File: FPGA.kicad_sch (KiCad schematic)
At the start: 1 part, among them U501 ICE40-HX8K_Breakout_Board

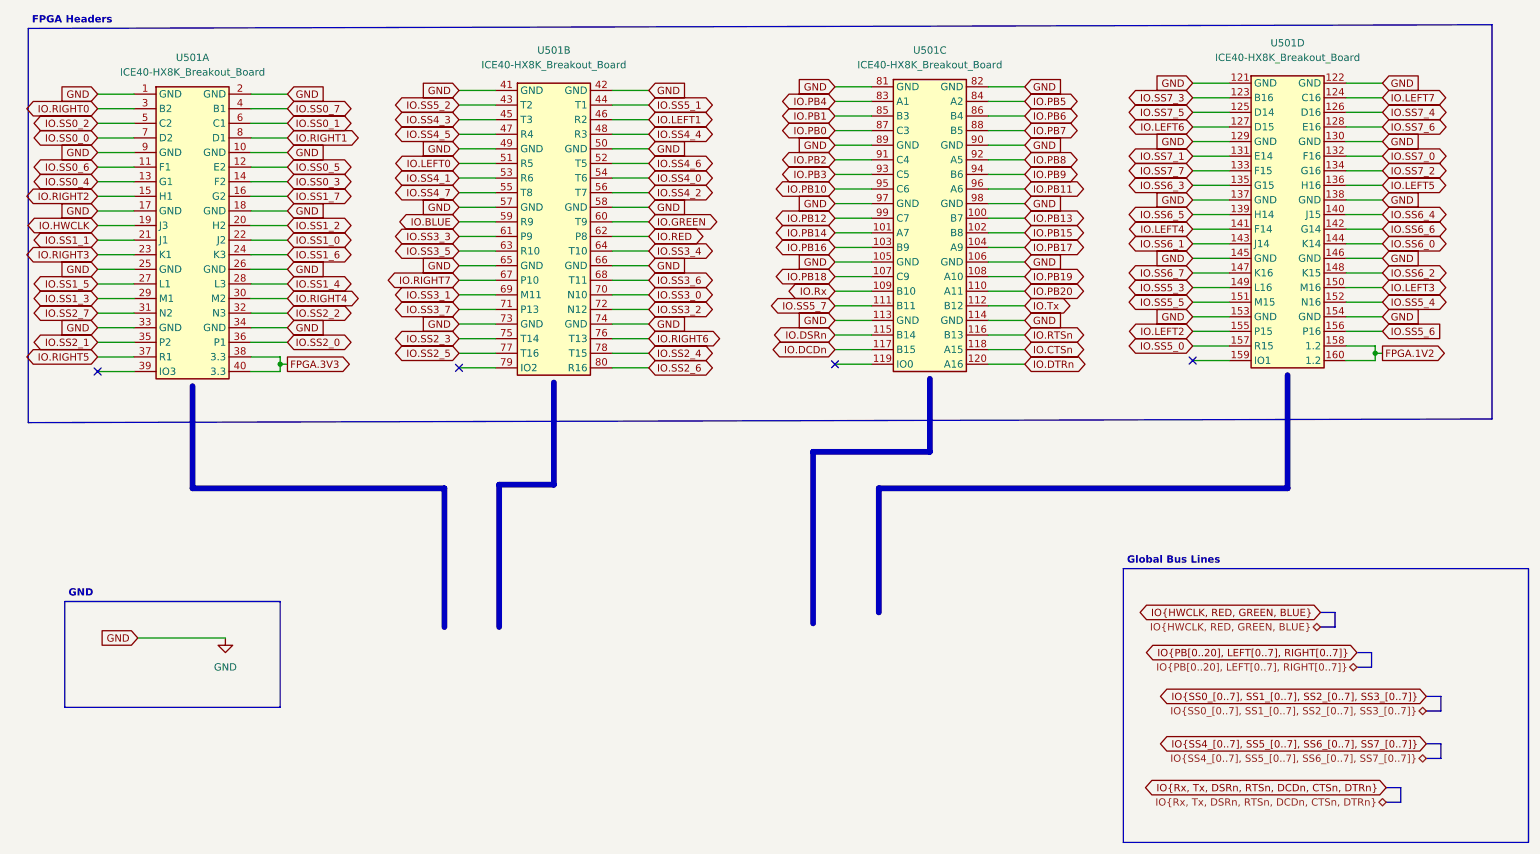
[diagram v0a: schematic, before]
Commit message: Complete Design
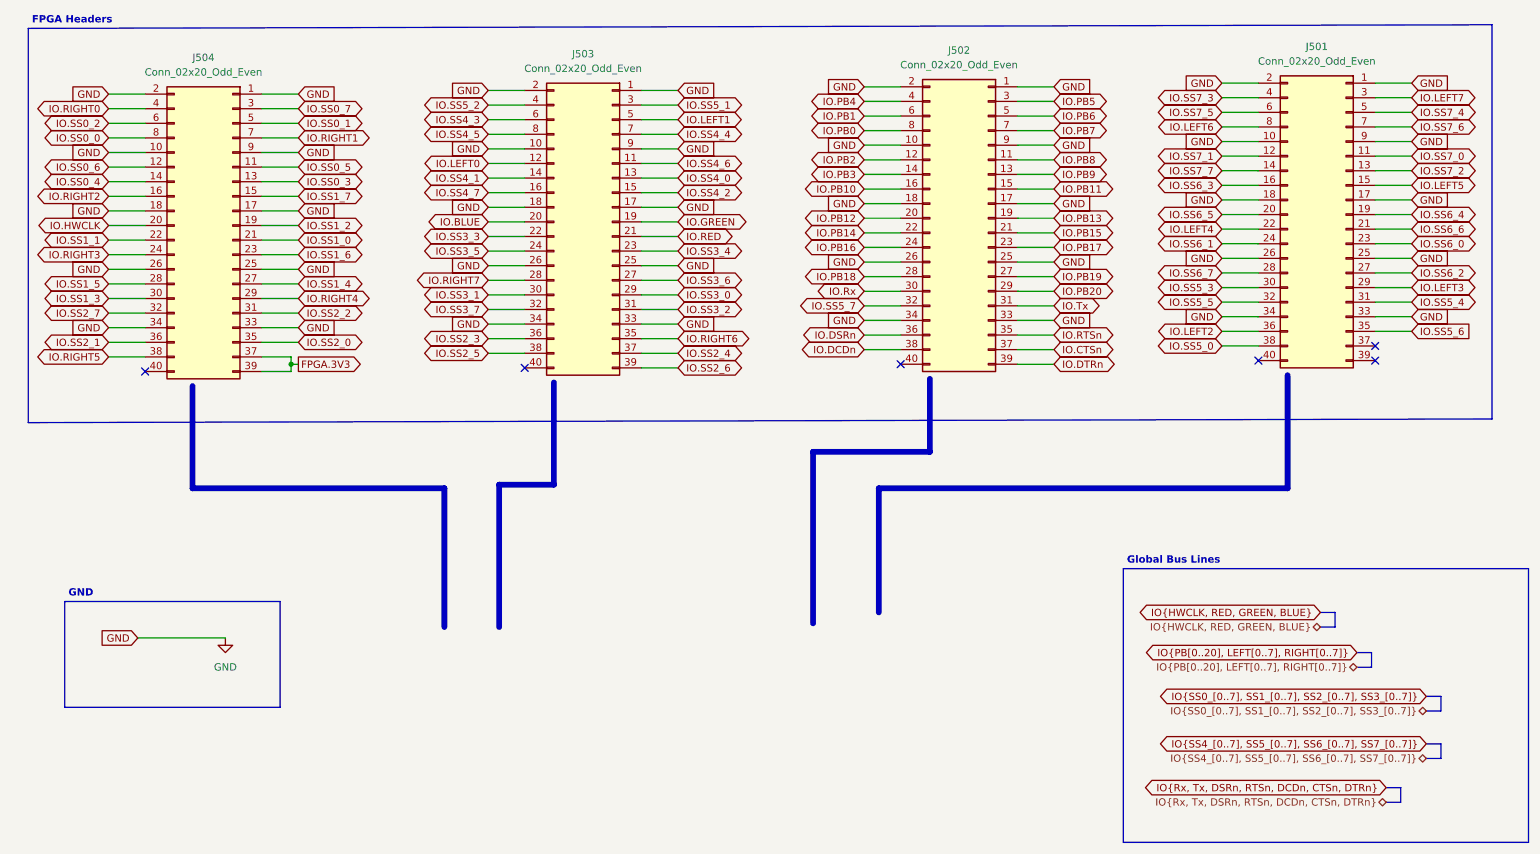
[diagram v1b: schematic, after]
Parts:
- removed U501: ICE40-HX8K_Breakout_Board, ECELab_Footprints:ICE40-HX8K Breakout Board, symbol ECELab_PartsLibrary:ICE40-HX8K_Breakout_Board
- added J501, J502, J503, J504: Conn_02x20_Odd_Even, Connector_PinHeader_2.54mm:PinHeader_2x20_P2.54mm_Vertical, symbol Connector_Generic:Conn_02x20_Odd_Even
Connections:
- net FPGA.3V3: now also J504.37 (Pin_37), J504.39 (Pin_39)
- net GND: now also J501.1 (Pin_1), J501.10 (Pin_10), J501.17 (Pin_17), J501.18 (Pin_18), J501.2 (Pin_2), J501.25 (Pin_25), J501.26 (Pin_26), J501.33 (Pin_33), J501.34 (Pin_34), J501.9 (Pin_9), J502.1 (Pin_1), J502.10 (Pin_10), J502.17 (Pin_17), J502.18 (Pin_18), J502.2 (Pin_2), J502.25 (Pin_25), J502.26 (Pin_26), J502.33 (Pin_33), J502.34 (Pin_34), J502.9 (Pin_9), J503.1 (Pin_1), J503.10 (Pin_10), J503.17 (Pin_17), J503.18 (Pin_18), J503.2 (Pin_2), J503.25 (Pin_25), J503.26 (Pin_26), J503.33 (Pin_33), J503.34 (Pin_34), J503.9 (Pin_9), J504.1 (Pin_1), J504.10 (Pin_10), J504.17 (Pin_17), J504.18 (Pin_18), J504.2 (Pin_2), J504.25 (Pin_25), J504.26 (Pin_26), J504.33 (Pin_33), J504.34 (Pin_34), J504.9 (Pin_9)
- net IO.BLUE: now also J503.20 (Pin_20)
- net IO.CTSn: now also J502.37 (Pin_37)
- net IO.DCDn: now also J502.38 (Pin_38)
- net IO.DSRn: now also J502.36 (Pin_36)
- net IO.DTRn: now also J502.39 (Pin_39)
- net IO.GREEN: now also J503.19 (Pin_19)
- net IO.HWCLK: now also J504.20 (Pin_20)
- net IO.LEFT0: now also J503.12 (Pin_12)
- net IO.LEFT1: now also J503.5 (Pin_5)
- net IO.LEFT2: now also J501.36 (Pin_36)
- net IO.LEFT3: now also J501.29 (Pin_29)
- net IO.LEFT4: now also J501.22 (Pin_22)
- net IO.LEFT5: now also J501.15 (Pin_15)
- net IO.LEFT6: now also J501.8 (Pin_8)
- net IO.LEFT7: now also J501.3 (Pin_3)
- net IO.PB0: now also J502.8 (Pin_8)
- net IO.PB1: now also J502.6 (Pin_6)
- net IO.PB10: now also J502.16 (Pin_16)
- net IO.PB11: now also J502.15 (Pin_15)
- net IO.PB12: now also J502.20 (Pin_20)
- net IO.PB13: now also J502.19 (Pin_19)
- net IO.PB14: now also J502.22 (Pin_22)
- net IO.PB15: now also J502.21 (Pin_21)
- net IO.PB16: now also J502.24 (Pin_24)
- net IO.PB17: now also J502.23 (Pin_23)
- net IO.PB18: now also J502.28 (Pin_28)
- net IO.PB19: now also J502.27 (Pin_27)
- net IO.PB2: now also J502.12 (Pin_12)
- net IO.PB20: now also J502.29 (Pin_29)
- net IO.PB3: now also J502.14 (Pin_14)
- net IO.PB4: now also J502.4 (Pin_4)
- net IO.PB5: now also J502.3 (Pin_3)
- net IO.PB6: now also J502.5 (Pin_5)
- net IO.PB7: now also J502.7 (Pin_7)
- net IO.PB8: now also J502.11 (Pin_11)
- net IO.PB9: now also J502.13 (Pin_13)
- net IO.RED: now also J503.21 (Pin_21)
- net IO.RIGHT0: now also J504.4 (Pin_4)
- net IO.RIGHT1: now also J504.7 (Pin_7)
- net IO.RIGHT2: now also J504.16 (Pin_16)
- net IO.RIGHT3: now also J504.24 (Pin_24)
- net IO.RIGHT4: now also J504.29 (Pin_29)
- net IO.RIGHT5: now also J504.38 (Pin_38)
- net IO.RIGHT6: now also J503.35 (Pin_35)
- net IO.RIGHT7: now also J503.28 (Pin_28)
- net IO.RTSn: now also J502.35 (Pin_35)
- net IO.Rx: now also J502.30 (Pin_30)
- net IO.SS0_0: now also J504.8 (Pin_8)
- net IO.SS0_1: now also J504.5 (Pin_5)
- net IO.SS0_2: now also J504.6 (Pin_6)
- net IO.SS0_3: now also J504.13 (Pin_13)
- net IO.SS0_4: now also J504.14 (Pin_14)
- net IO.SS0_5: now also J504.11 (Pin_11)
- net IO.SS0_6: now also J504.12 (Pin_12)
- net IO.SS0_7: now also J504.3 (Pin_3)
- net IO.SS1_0: now also J504.21 (Pin_21)
- net IO.SS1_1: now also J504.22 (Pin_22)
- net IO.SS1_2: now also J504.19 (Pin_19)
- net IO.SS1_3: now also J504.30 (Pin_30)
- net IO.SS1_4: now also J504.27 (Pin_27)
- net IO.SS1_5: now also J504.28 (Pin_28)
- net IO.SS1_6: now also J504.23 (Pin_23)
- net IO.SS1_7: now also J504.15 (Pin_15)
- net IO.SS2_0: now also J504.35 (Pin_35)
- net IO.SS2_1: now also J504.36 (Pin_36)
- net IO.SS2_2: now also J504.31 (Pin_31)
- net IO.SS2_3: now also J503.36 (Pin_36)
- net IO.SS2_4: now also J503.37 (Pin_37)
- net IO.SS2_5: now also J503.38 (Pin_38)
- net IO.SS2_6: now also J503.39 (Pin_39)
- net IO.SS2_7: now also J504.32 (Pin_32)
- net IO.SS3_0: now also J503.29 (Pin_29)
- net IO.SS3_1: now also J503.30 (Pin_30)
- net IO.SS3_2: now also J503.31 (Pin_31)
- net IO.SS3_3: now also J503.22 (Pin_22)
- net IO.SS3_4: now also J503.23 (Pin_23)
- net IO.SS3_5: now also J503.24 (Pin_24)
- net IO.SS3_6: now also J503.27 (Pin_27)
- net IO.SS3_7: now also J503.32 (Pin_32)
- net IO.SS4_0: now also J503.13 (Pin_13)
- net IO.SS4_1: now also J503.14 (Pin_14)
- net IO.SS4_2: now also J503.15 (Pin_15)
- net IO.SS4_3: now also J503.6 (Pin_6)
- net IO.SS4_4: now also J503.7 (Pin_7)
- net IO.SS4_5: now also J503.8 (Pin_8)
- net IO.SS4_6: now also J503.11 (Pin_11)
- net IO.SS4_7: now also J503.16 (Pin_16)
- net IO.SS5_0: now also J501.38 (Pin_38)
- net IO.SS5_1: now also J503.3 (Pin_3)
- net IO.SS5_2: now also J503.4 (Pin_4)
- net IO.SS5_3: now also J501.30 (Pin_30)
- net IO.SS5_4: now also J501.31 (Pin_31)
- net IO.SS5_5: now also J501.32 (Pin_32)
- net IO.SS5_6: now also J501.35 (Pin_35)
- net IO.SS5_7: now also J502.32 (Pin_32)
- net IO.SS6_0: now also J501.23 (Pin_23)
- net IO.SS6_1: now also J501.24 (Pin_24)
- net IO.SS6_2: now also J501.27 (Pin_27)
- net IO.SS6_3: now also J501.16 (Pin_16)
- net IO.SS6_4: now also J501.19 (Pin_19)
- net IO.SS6_5: now also J501.20 (Pin_20)
- net IO.SS6_6: now also J501.21 (Pin_21)
- net IO.SS6_7: now also J501.28 (Pin_28)
- net IO.SS7_0: now also J501.11 (Pin_11)
- net IO.SS7_1: now also J501.12 (Pin_12)
- net IO.SS7_2: now also J501.13 (Pin_13)
- net IO.SS7_3: now also J501.4 (Pin_4)
- net IO.SS7_4: now also J501.5 (Pin_5)
- net IO.SS7_5: now also J501.6 (Pin_6)
- net IO.SS7_6: now also J501.7 (Pin_7)
- net IO.SS7_7: now also J501.14 (Pin_14)
- net IO.Tx: now also J502.31 (Pin_31)
- no-connect marks 4 -> 6
